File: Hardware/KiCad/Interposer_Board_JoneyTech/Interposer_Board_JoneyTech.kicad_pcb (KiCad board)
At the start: 2 copper layers, 123 x 99.5 mm, 6 parts, among them J1 M.2 Key M, J2 M.2 Key M

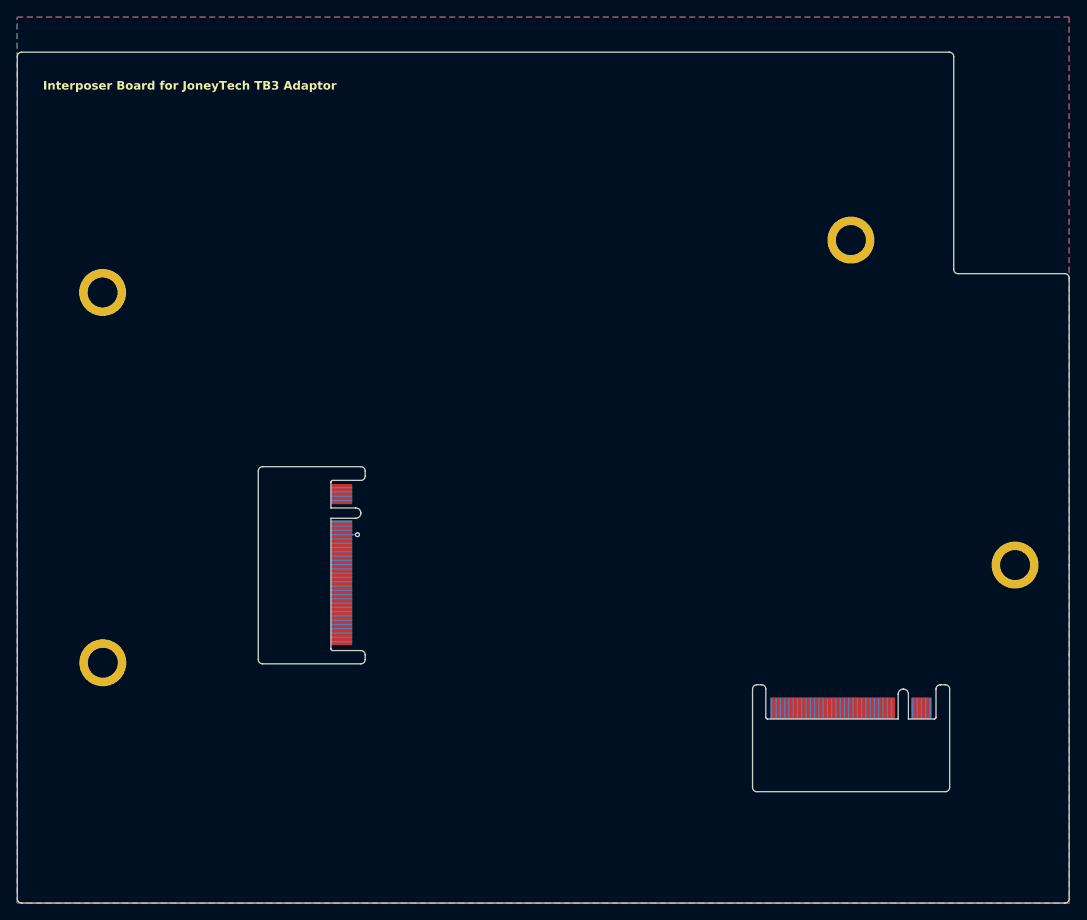
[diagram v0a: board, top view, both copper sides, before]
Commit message: Reduced Board Length from 123mm to 122.5mm
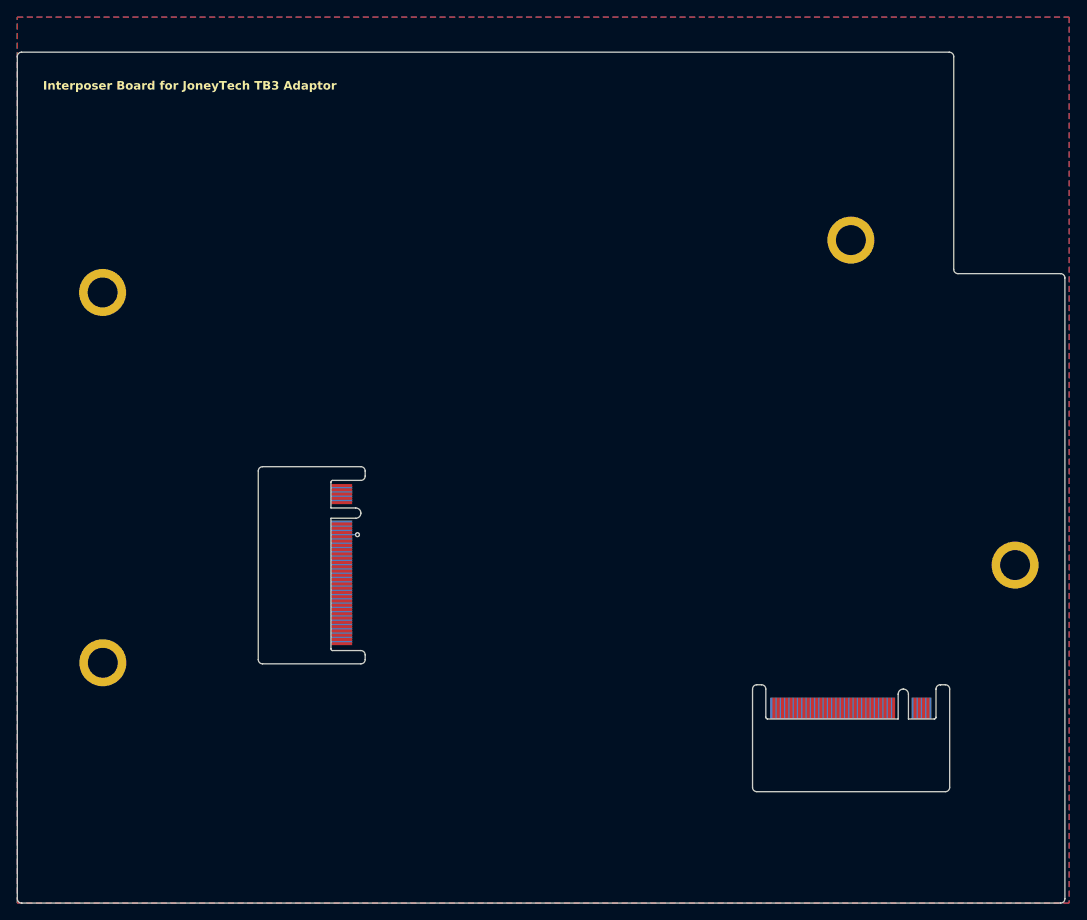
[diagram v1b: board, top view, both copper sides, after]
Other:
- board size 123 x 99.5 mm -> 122.5 x 99.5 mm
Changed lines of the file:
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@@
 	)
 	(gr_arc
-		(start 192.2761 46.2786)
-		(mid 192.629653 46.425047)
-		(end 192.7761 46.7786)
+		(start 191.7761 46.2786)
+		(mid 192.129653 46.425047)
+		(end 192.2761 46.7786)
 		(stroke
 			(width 0.05)
@@
 			(width 0.05)
 			(type solid)
-		)
-		(layer "Edge.Cuts")
-	)
-	(gr_line
-		(start 192.7761 90.8536)
-		(end 192.7761 119.3786)
-		(stroke
-			(width 0.05)
-			(type default)
 		)
 		(layer "Edge.Cuts")
@@
 	)
 	(gr_arc
-		(start 192.7761 119.3786)
-		(mid 192.629653 119.732153)
-		(end 192.2761 119.878601)
+		(start 192.2761 119.3786)
+		(mid 192.129653 119.732153)
+		(end 191.7761 119.878601)
 		(stroke
 			(width 0.05)
@@
 		(layer "Edge.Cuts")
 	)
+	(gr_arc
+		(start 70.2761 119.8786)
+		(mid 69.922547 119.732153)
+		(end 69.7761 119.3786)
+		(stroke
+			(width 0.05)
+			(type default)
+		)
+		(layer "Edge.Cuts")
+	)
 	(gr_line
 		(start 109.9511 91.903601)
@@
 			(width 0.05)
 			(type default)
-		)
-		(layer "Edge.Cuts")
-	)
-	(gr_arc
-		(start 70.2761 119.8786)
-		(mid 69.922546 119.732153)
-		(end 69.7761 119.378599)
-		(stroke
-			(width 0.05)
-			(type solid)
 		)
 		(layer "Edge.Cuts")
@@
 	(gr_line
 		(start 179.7761 46.2786)
-		(end 192.2761 46.278599)
+		(end 191.7761 46.2786)
 		(stroke
 			(width 0.05)
@@
 	)
 	(gr_line
-		(start 192.7761 80.3536)
-		(end 192.7761 90.8536)
-		(stroke
-			(width 0.05)
-			(type default)
-		)
-		(layer "Edge.Cuts")
-	)
-	(gr_line
 		(start 106.4511 74.8786)
 		(end 106.4511 90.1536)
@@
 	)
 	(gr_line
-		(start 192.7761 80.3536)
-		(end 192.7761 46.7786)
-		(stroke
-			(width 0.05)
-			(type default)
-		)
-		(layer "Edge.Cuts")
-	)
-	(gr_line
-		(start 192.2761 119.878601)
+		(start 191.7761 119.8786)
 		(end 70.2761 119.8786)
 		(stroke
@@
 	(gr_line
 		(start 69.7761 119.3786)
-		(end 69.776105 20.8786)
+		(end 69.7761 20.8786)
 		(stroke
 			(width 0.05)
@@
 		)
 		(layer "Edge.Cuts")
+	)
+	(gr_line
+		(start 192.2761 119.3786)
+		(end 192.2761 46.7786)
+		(stroke
+			(width 0.05)
+			(type default)
+		)
+		(layer "Edge.Cuts")
